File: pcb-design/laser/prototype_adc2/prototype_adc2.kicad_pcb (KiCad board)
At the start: 4 copper layers, 37 x 26 mm, 59 parts, among them J1 Conn_01x01_Socket, J2 Conn_01x01_Socket, J3 Conn_01x01_Socket, J4 Conn_01x01_Socket, J5 Conn_01x01_Socket, J6 Conn_01x01_Socket, J7 Conn_01x01_Socket, J8 Conn_01x01_Socket, J9 Conn_01x01_Socket, U2 MCP1541T-I_TT, U3 MEA1D2409SC

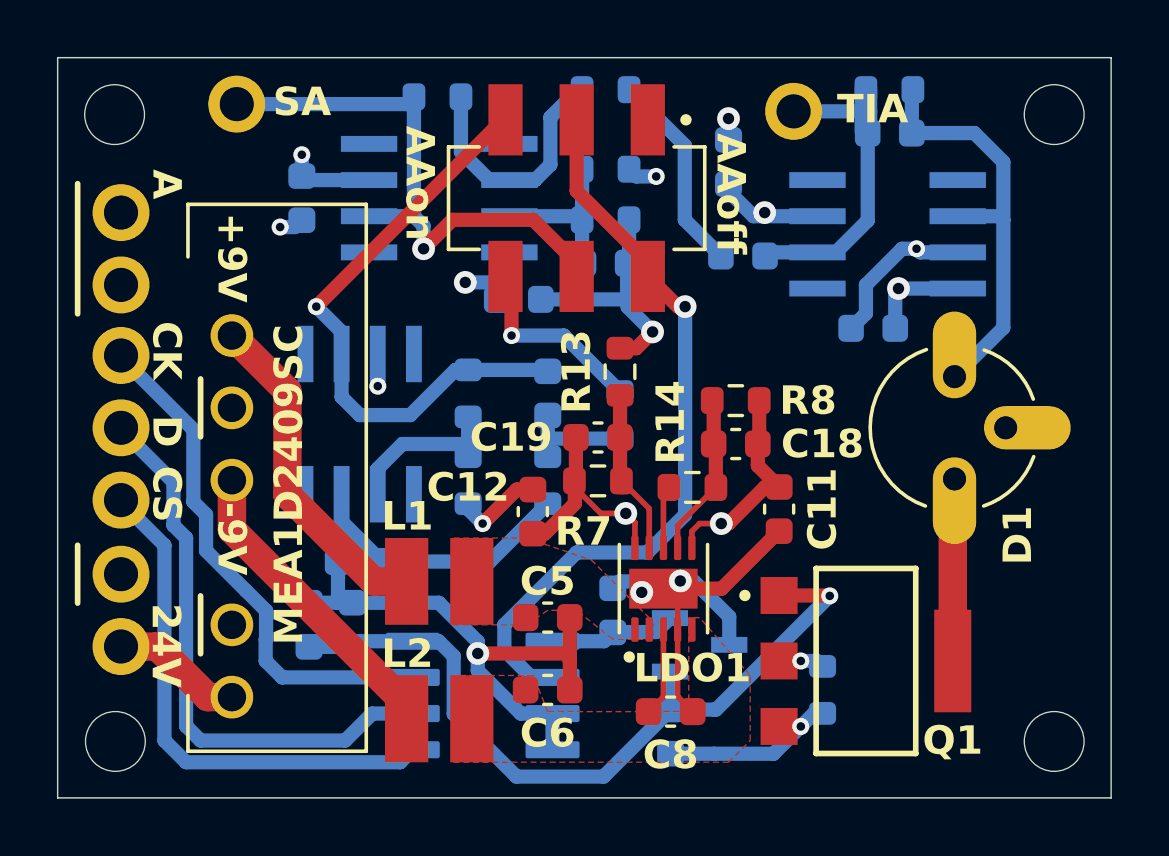
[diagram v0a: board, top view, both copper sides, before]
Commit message: fixed laser footprint on pcb
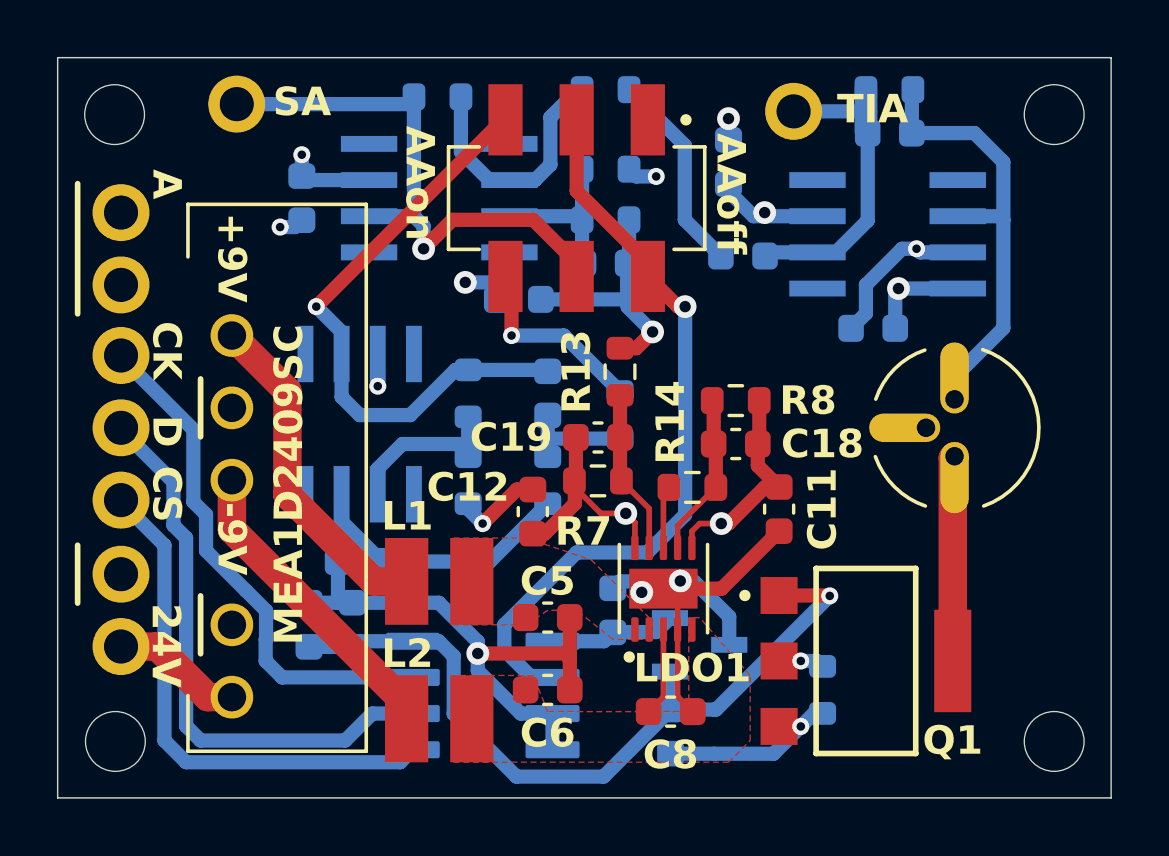
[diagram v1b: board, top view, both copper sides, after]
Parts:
- D1: moved to B.Cu
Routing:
- net /ld_i: track 6.42 -> 8.01 mm
- net /pd_out: track 15.1 -> 15.9 mm
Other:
- board text removed: "FIX LASER FOOTPRINT"
